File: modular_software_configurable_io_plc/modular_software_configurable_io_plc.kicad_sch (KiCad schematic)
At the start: 23 parts, among them J1 FW-14-03-G-D-085-155, J10 CLP-108-02-G-D-BE, J11 CLP-102-02-G-D-BE, J12 CLP-102-02-G-D-BE, J13 CLP-102-02-G-D-BE, J14 CLP-108-02-G-D-BE, J15 FW-14-03-G-D-085-155, J16 FW-02-03-G-D-085-155, J17 FW-02-03-G-D-085-155, J18 FW-02-03-G-D-085-155, J19 FW-02-03-G-D-085-155, J2 CLP-102-02-G-D-BE, J3 CLP-102-02-G-D-BE, J4 CLP-104-02-G-D-BE, J5 CLP-104-02-G-D-BE, J6 CLP-102-02-G-D-BE, J7 CLP-102-02-G-D-BE, J8 CLP-114-02-G-D-BE, J9 CLP-102-02-G-D-BE

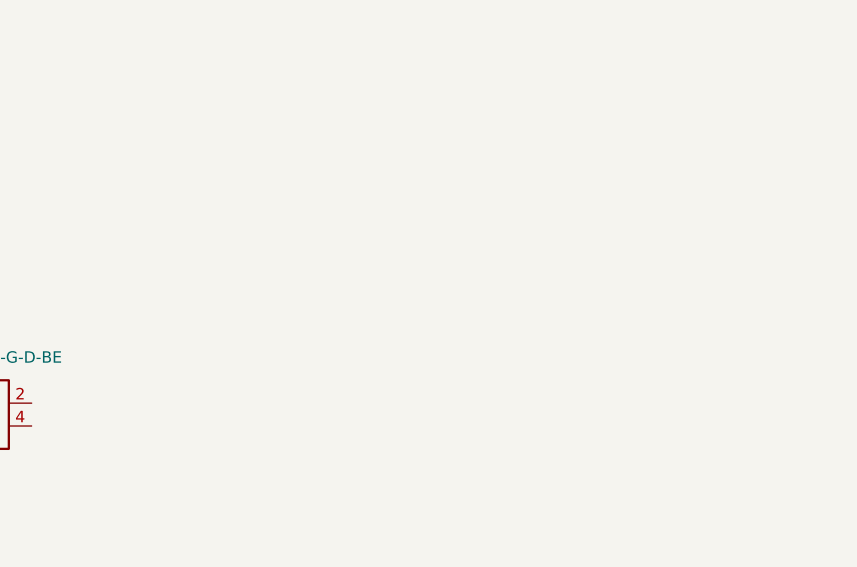
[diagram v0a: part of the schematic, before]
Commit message: Backup
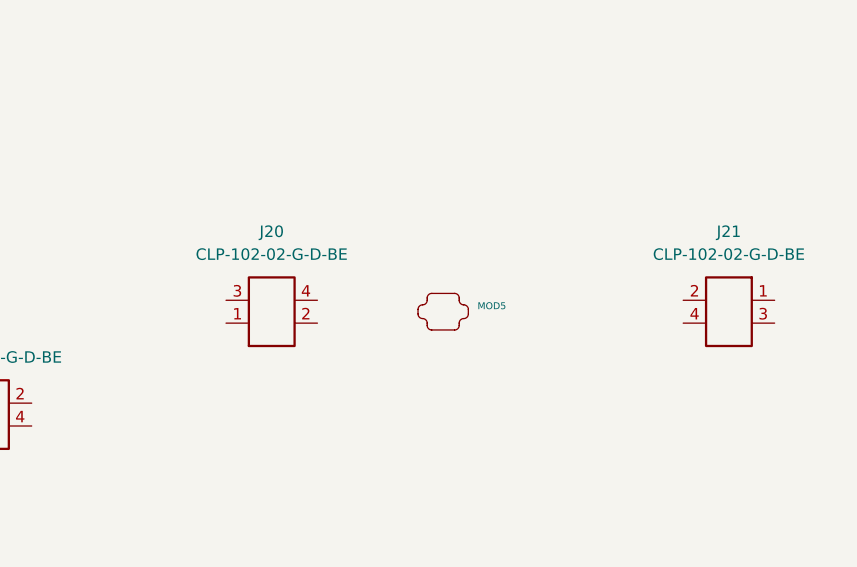
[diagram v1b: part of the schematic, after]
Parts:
- added J20, J21: CLP-102-02-G-D-BE, connector_footprints:CLP-102-02-G-D-BE, symbol UNITED_CONNECTORS_DATA_BASE:J_CLP-102-02-G-D-BE
- added MOD5: ~, modules_footprints:minimal_ltc9111, symbol UNITED_MODULES_DATA_BASE:MINIMAL_LTC9111

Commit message: Backup
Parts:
- MOD3, MOD5: 3dviewer Link (none) -> https://3dviewer.net/index.html#model=https://github.com/io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
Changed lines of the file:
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@@
+			)
+		)
+		(property "3dviewer Link" "https://3dviewer.net/index.html#model=https://github.com/ionutms/KiCAD_Symbols_Generator/blob/main/3D_models/minimal_adp1032.wrl"
+			(at 227.33 123.19 0)
+			(effects
+				(font
+					(size 1.27 1.27)
+				)
+				(justify left)
+				(hide yes)
 			)
 		)
@@
 				(hide yes)
 			)
+		)
+		(property "3dviewer Link" "https://3dviewer.net/index.html#model=https://github.com/ionutms/KiCAD_Symbols_Generator/blob/main/3D_models/minimal_ltc9111.wrl"
+			(at 323.85 83.82 0)
+			(effects
+				(font
+					(size 1.27 1.27)
+				)
+				(justify left)
+				(hide yes)
+			)

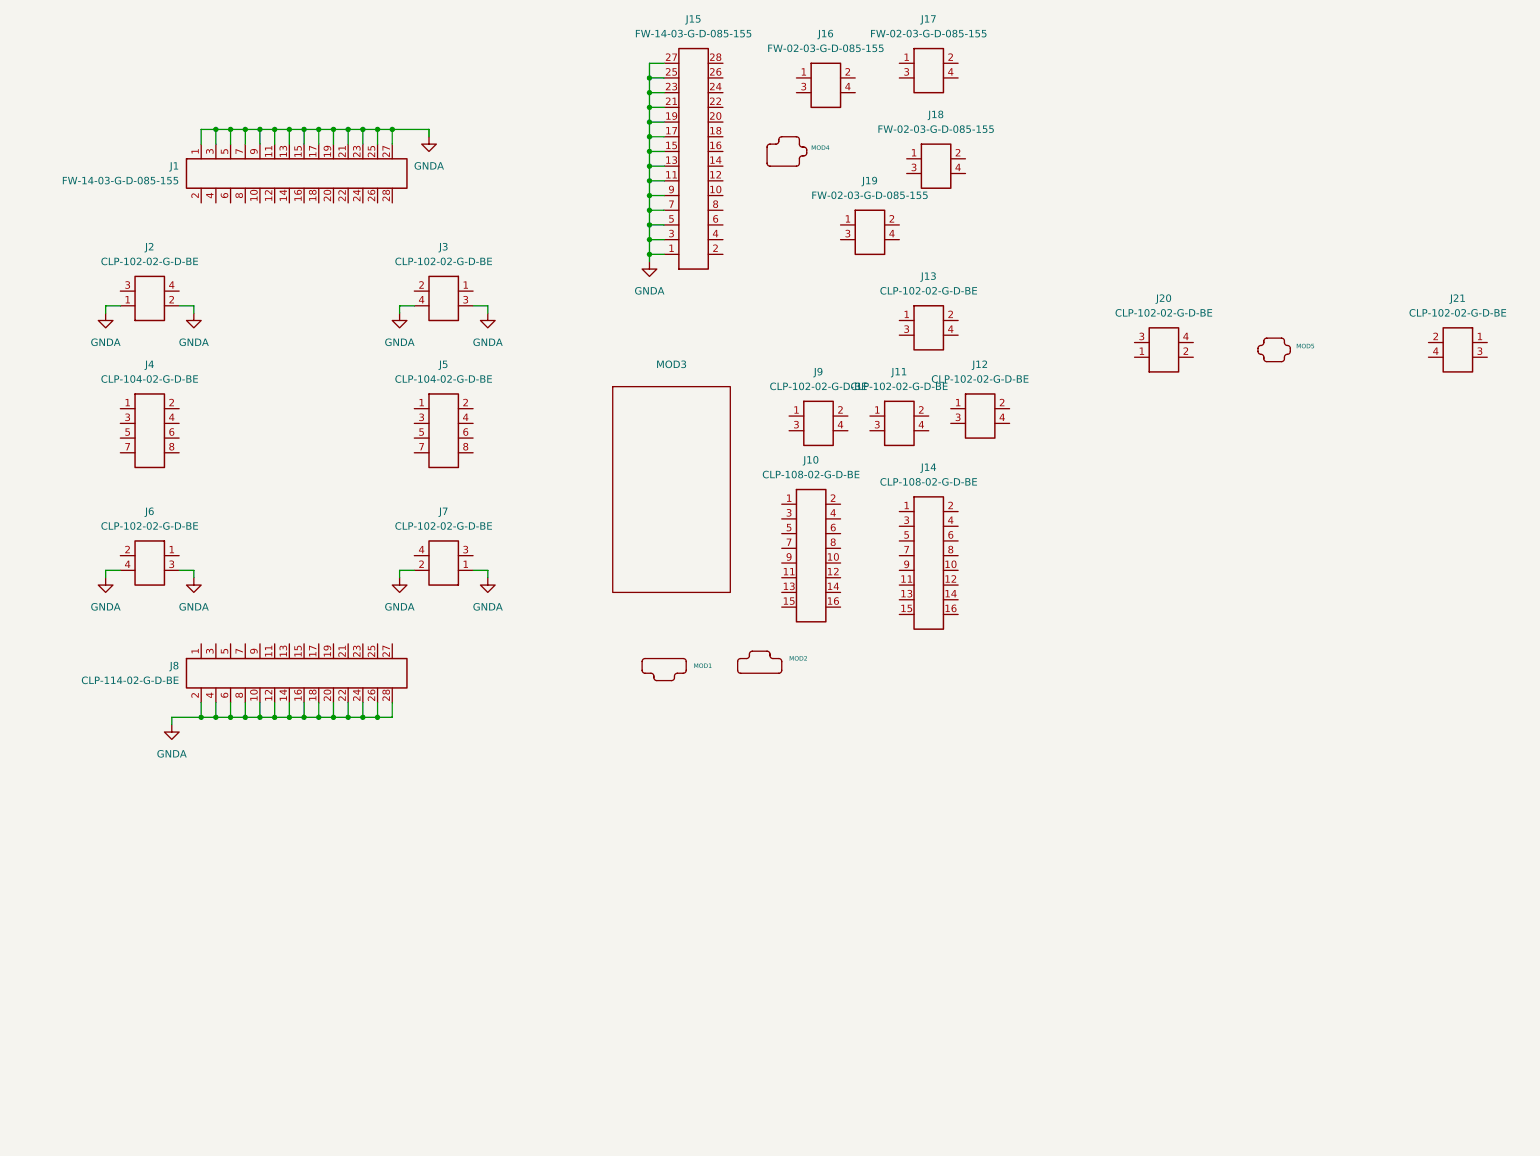
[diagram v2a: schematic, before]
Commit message: Backup
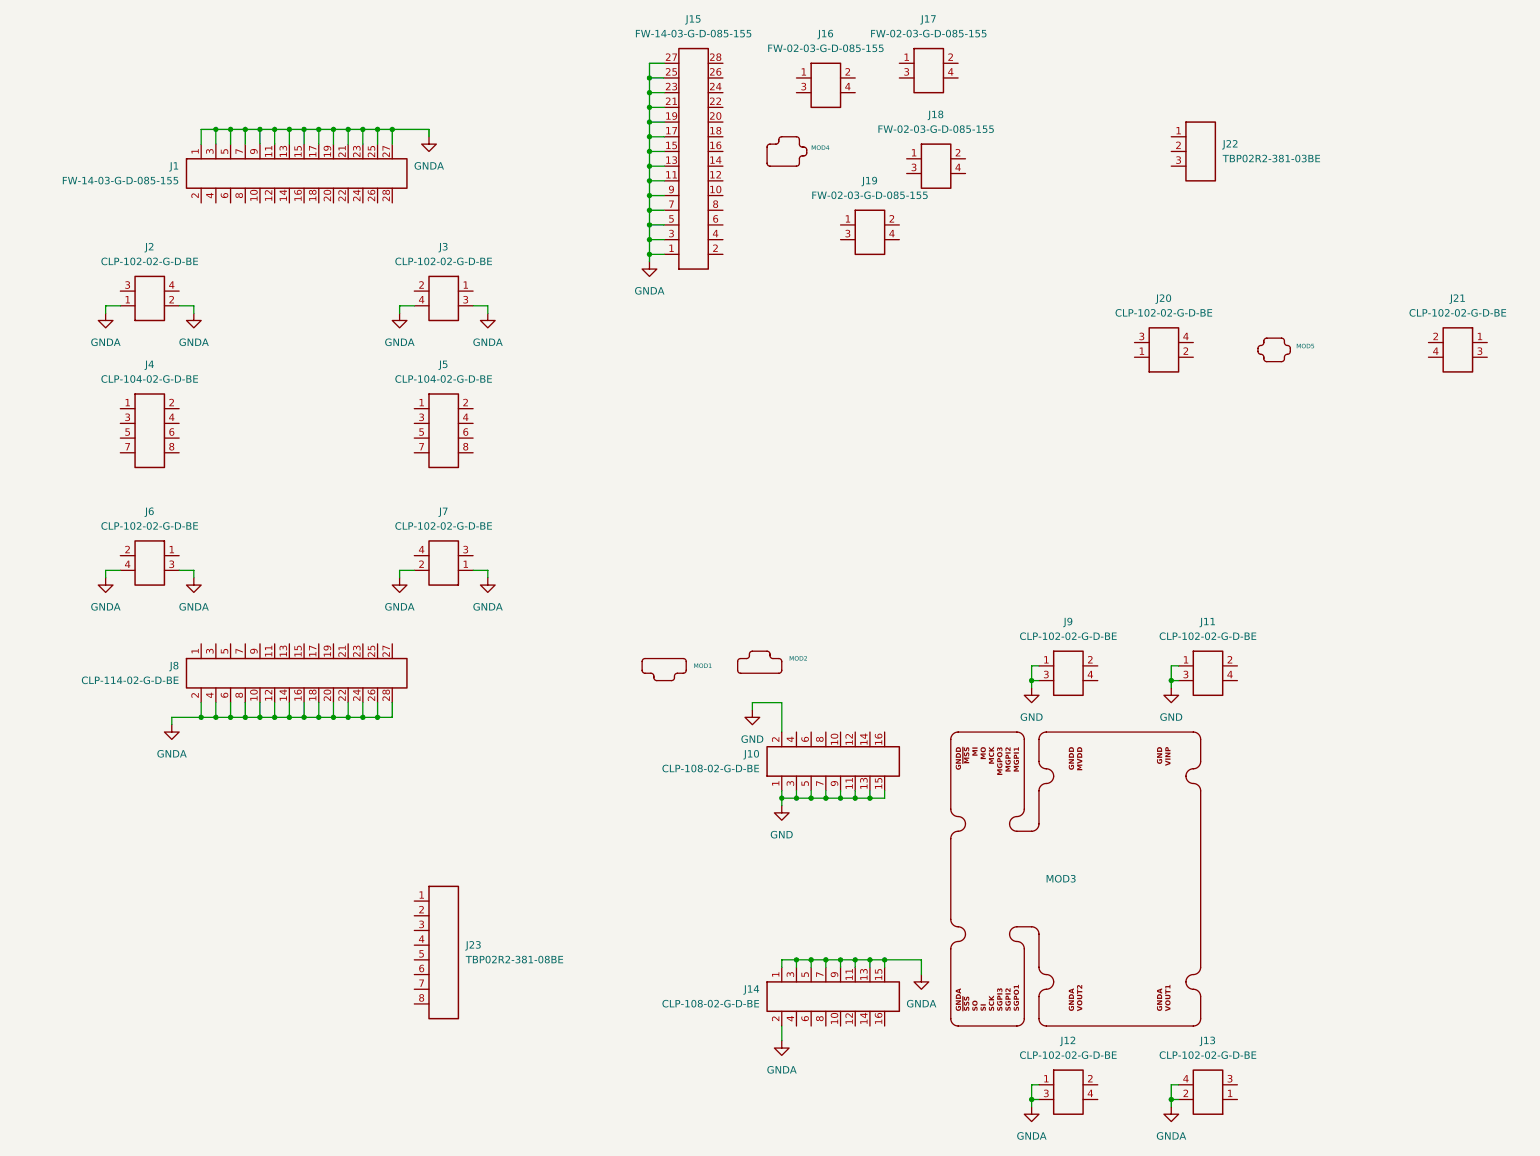
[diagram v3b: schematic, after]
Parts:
- added J22: TBP02R2-381-03BE, connector_footprints:TBP02R2-381-03BE, symbol UNITED_CONNECTORS_DATA_BASE:J_TBP02R2-381-03BE
- added J23: TBP02R2-381-08BE, connector_footprints:TBP02R2-381-08BE, symbol UNITED_CONNECTORS_DATA_BASE:J_TBP02R2-381-08BE
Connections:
- net GNDA: now also J12.1, J12.3, J13.2, J13.4, J14.1, J14.11, J14.13, J14.15, J14.2, J14.3, J14.5, J14.7, J14.9
- net GND: now reaches J10.1
- net GND: now also J10.11, J10.13, J10.15, J10.2, J10.3, J10.5, J10.7, J10.9, J11.1, J11.3, J9.1, J9.3
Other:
- moved on the sheet: J10, J11, J12, J13, J14, J9
